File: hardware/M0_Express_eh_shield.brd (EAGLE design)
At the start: 51.3 x 53.3 mm, 35 parts, among them U1 TLV3691, U2 AB0815, U3 Value, U4 MIC841, U5 TPS781, U6 ISL21080, X2 ABS05-32.768KHZ-9-T

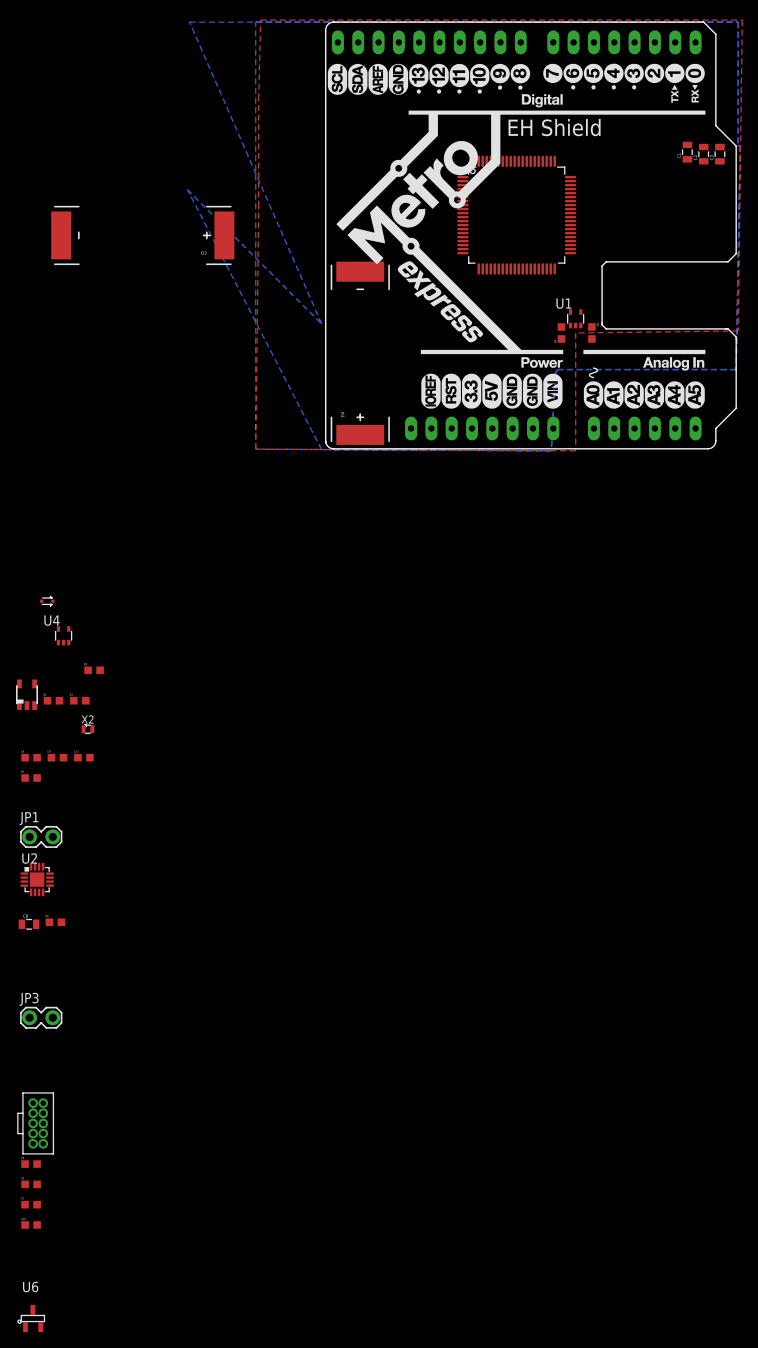
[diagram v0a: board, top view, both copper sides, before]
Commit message: finished hardware
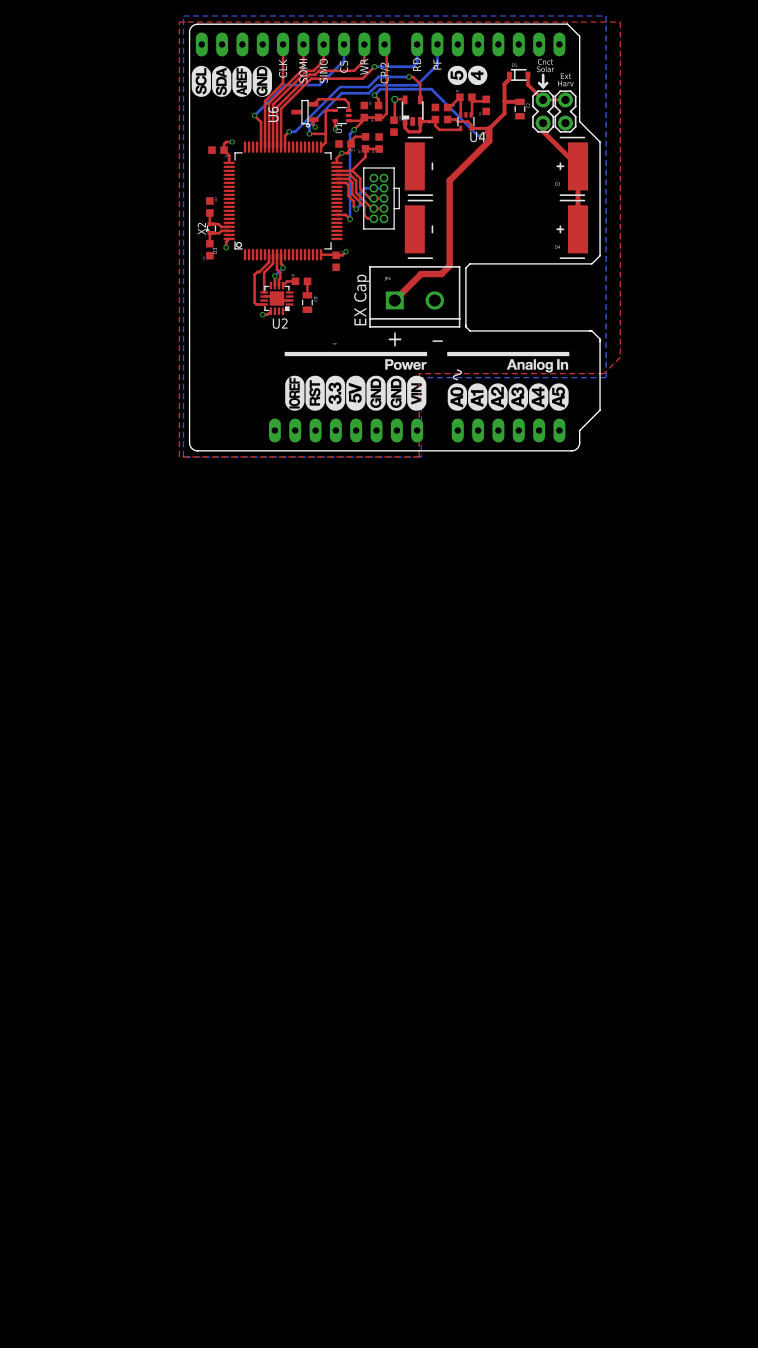
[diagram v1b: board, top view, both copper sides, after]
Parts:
- removed C1, C3: (no value), SparkFun-Capacitors:0805
- added C11: 0.1u, tiny_passives:0603
- added JP4: (no value), SparkFun-Connectors:SCREWTERMINAL-5MM-2
- C2: value (none) -> 10u
- D1: value RB751 -> BAT20JFILM; device SparkFun-DiscreteSemi:SOD-523 -> SparkFun-DiscreteSemi:SOD-323
- moved U6 154.6 mm to (14.7, 42.1), turned to 90 degrees
- moved C10 144.7 mm to (25.8, 40.3), turned to 270 degrees
- moved C6 143.1 mm to (31.0, 41.9), turned to 90 degrees
- moved JP3 129.0 mm to (44.5, 40.9), turned to 90 degrees
- moved C5 128.9 mm to (3.81, 37.3), turned to 180 degrees
- moved C7 123.9 mm to (18.6, 23.4), turned to 270 degrees
- moved JP2 118.9 mm to (24.6, 28.8), turned to 180 degrees
- moved JP1 111.6 mm to (47.2, 40.9), turned to 90 degrees
- moved R7 89.7 mm to (22.3, 38.3), turned to 90 degrees
- moved R2 89.6 mm to (34.8, 43.9)
- moved R1 88.4 mm to (32.5, 41.9), turned to 270 degrees
- moved D1 88.3 mm to (41.4, 46.7)
- moved C4 88.3 mm to (24.0, 38.2), turned to 90 degrees
- moved U5 87.5 mm to (28.1, 42.3)
- moved R3 86.0 mm to (37.3, 42.9), turned to 90 degrees
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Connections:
- removed net D6: IOL.2
- removed net D7: IOL.1
- net GND: now also C11.2, JP4.2; no longer C1.2, C3.2
- net NV_READ: now also IOL.1, U3.51; no longer IOH.10, U3.52
- net NV_WRITE: now also U3.52; no longer U3.51
- net PFAIL: now also IOL.2, U3.41; no longer AD.5, U3.2
- net REG_SET: now also U3.50; no longer U3.3
- net RTC_CE: now also U3.7; no longer U3.26
- net RTC_SCLK: now also U3.10; no longer U3.25
- net RTC_SIMO: now also U3.8; no longer U3.13
- net RTC_SOMI: now also U3.9; no longer U3.14
- net RX_DEBUG: now also U3.36; no longer U3.42
- net TX_DEBUG: now also U3.35; no longer U3.41
- net VCAP: now also JP4.1; no longer C1.1, C3.1
- net VCAP_HALF: now also IOH.10, U3.27; no longer AD.6, U3.1
- net VCC: now also C11.1
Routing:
- net VCAP: track 0.00 -> 62.9 mm, vias 0 -> 2
- net PFAIL: track 0.00 -> 30.7 mm, vias 0 -> 1
- net VCAP_HALF: track 0.00 -> 28.8 mm, vias 0 -> 2
- net NV_READ: track 0.00 -> 26.5 mm, vias 0 -> 1
- net REG_SET: track 0.00 -> 23.7 mm, vias 0 -> 2
- net VCC: track 0.00 -> 21.7 mm, vias 0 -> 8
- net NV_WRITE: track 0.00 -> 20.3 mm
- net NV_CS: track 0.00 -> 20.3 mm, vias 0 -> 1
- net NV_SIMO: track 0.00 -> 15.9 mm
- net N$10: track 0.00 -> 15.1 mm
- net NV_SOMI: track 0.00 -> 14.6 mm
- net NV_CLK: track 0.00 -> 13.8 mm
- net MSP430_RST: track 0.00 -> 13.3 mm
- net TX_DEBUG: track 0.00 -> 10.4 mm, vias 0 -> 1
- net N$7: track 0.00 -> 10.3 mm
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- added copper zone on layer 16, net VCC
- removed copper zone on layer 16, net GND
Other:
- outline, holes or cut-outs redrawn
- board text added: "+"
- board text added: "CLK"
- board text added: "CP/2"
- board text added: "CS"
- board text added: "Cnct Solar"
- board text added: "EX Cap"
- board text added: "Ext Harv"
- board text added: "PF"
- board text added: "RD"
- board text added: "SIMO"
- board text added: "SOMI"
- board text added: "WR"
- board text added: "_"
- board text removed: "EH Shield"
